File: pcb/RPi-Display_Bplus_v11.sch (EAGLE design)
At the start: 59 parts, among them IC1 ADS7846, IC2 24LC32A, IC3 LDO-TS9011-3V3, Q1 N-CHN, SW1 SWITCH-PTS840P, SW2 SWITCH-PTS840P, SW3 SWITCH-PTS840P, X1 PASSER, X2 PASSER, X3 PASSER, X4 PASSER

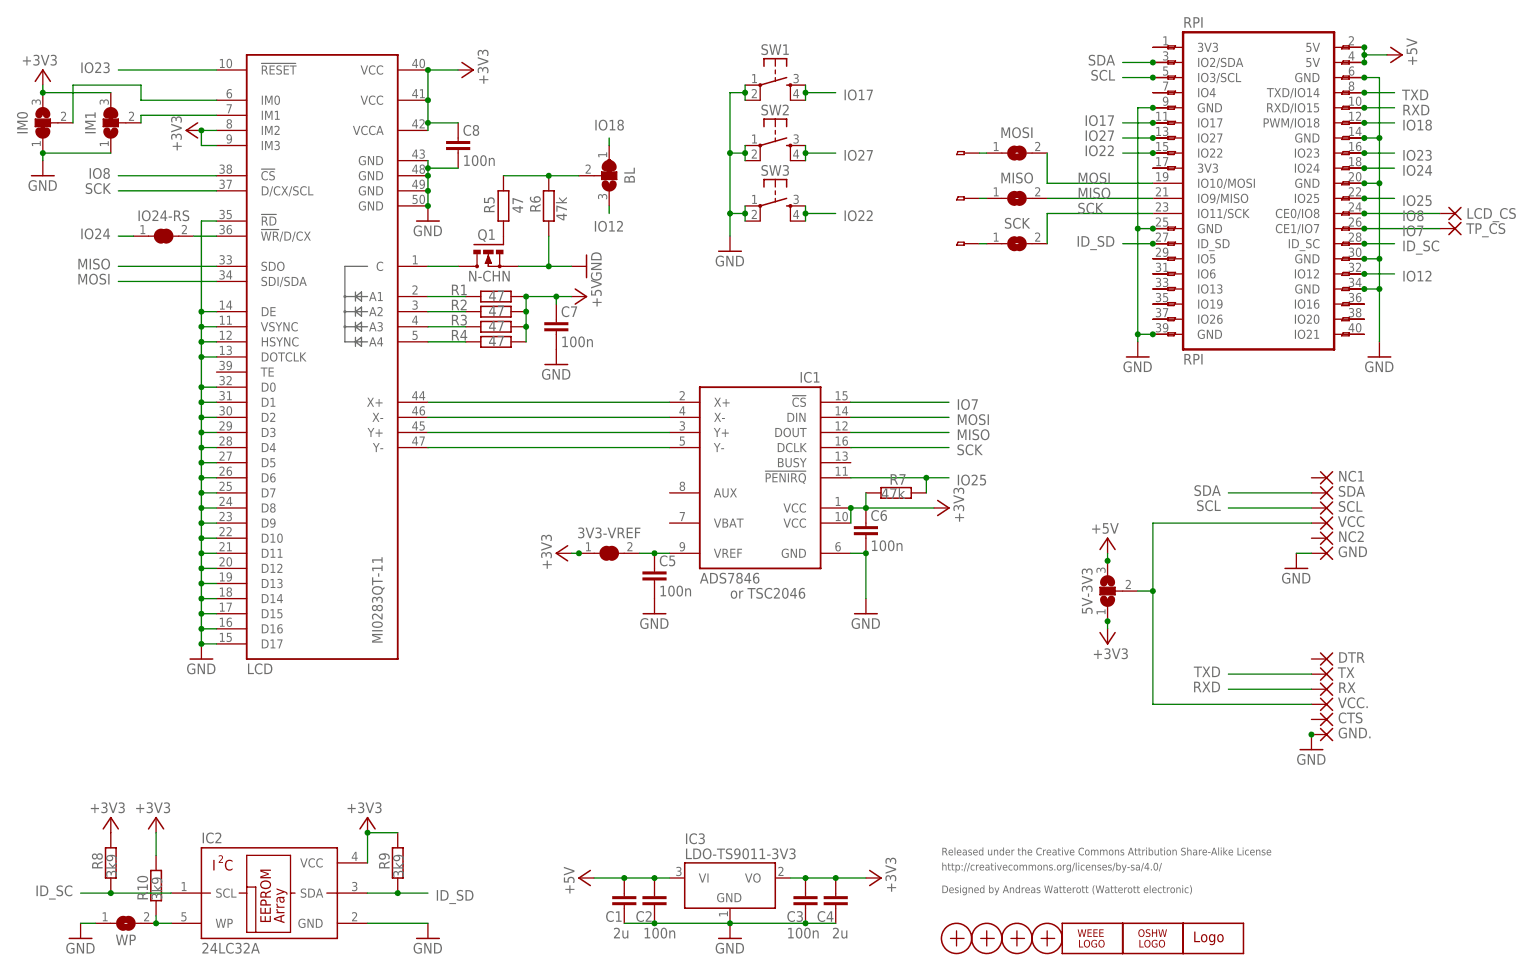
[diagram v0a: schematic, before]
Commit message: updated layout and schematics
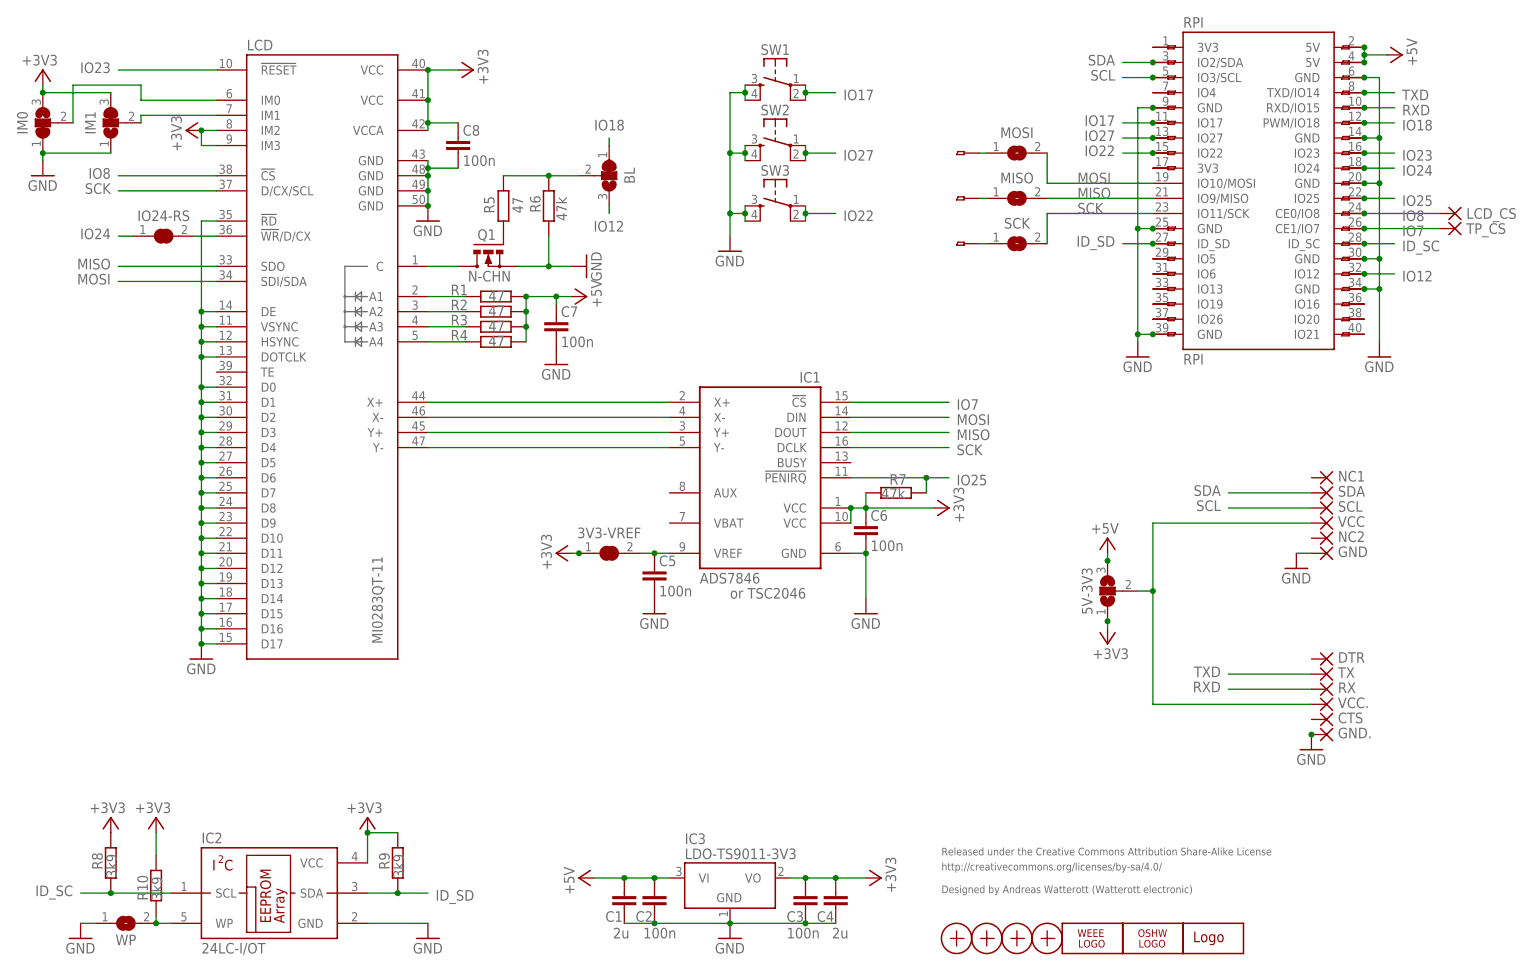
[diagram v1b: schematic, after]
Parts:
- 3V3-VREF, IO24-RS, MISO, MOSI, SCK, WP: value JUMPER2-NOCREAM -> JUMPER2-0603-NC; device we-rcl:JUMPER2-NOCREAM -> we-rcl:JUMPER2-0603-NC
- 5V-3V3, BL, IM0, IM1: value JUMPER3-NOCREAM -> JUMPER3-0603-NC; device we-rcl:JUMPER3-NOCREAM -> we-rcl:JUMPER3-0603-NC
- IC2: value 24LC32A -> 24LC-I/OT; device we-chip:I2C_EEPROM-CAT24AA0X -> we-chip:24LC-I/OT
- LOGO2: value WEEE_LOGO -> WEEE_LOGO-M; device we-symbol:WEEE_LOGO -> we-symbol:WEEE_LOGO-M
- RPI: device we-board:RPI_B+ -> we-board:RPI_B+-CON
- SW1, SW2, SW3: value SWITCH-PTS840P -> SW-TACTILE-PTS840P; device we-switch:SWITCH-PTS840P -> we-switch:SW-TACTILE-PTS840P
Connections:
- net GND: now also SW1.S1, SW1.S2, SW2.S1, SW2.S2, SW3.S1, SW3.S2; no longer SW1.P, SW1.P1, SW2.P, SW2.P1, SW3.P, SW3.P1
- net IO17: now also SW1.P1, SW1.P2; no longer SW1.S, SW1.S1
- net IO22: now also SW3.P1, SW3.P2; no longer SW3.S, SW3.S1
- net IO27: now also SW2.P1, SW2.P2; no longer SW2.S, SW2.S1
